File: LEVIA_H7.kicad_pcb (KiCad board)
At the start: 6 copper layers, 36.7 x 36.7 mm, 145 parts, among them J1 TF-028-H265, Q1 AO3400A, SW1 SW_Push, U1 USBLC6-2P6, U10 ZX-SH1.0-4PWT, U11 ZX-SH1.0-3PWT, U12 SIT1051TK/3, U13 ZX-SH1.0-4PWT, U14 ICM-42688-P, U15 ICM-42688-P, U16 DPS368XTSA1, U17 IST8310, U18 ZX-SH1.0-4PWT, U19 ZX-SH1.0-6PWT, U2 STM32H743VIHx, U20 ZX-SH1.0-6PWT, U21 ZX-SH1.0-3PWT, U22 ZX-SH1.0-8PWT, U24 ZX-SH1.0-4PWT, U25 BME680, U3 ZX-SH1.0-4PWT, U4 LMR43620R5RPER, U5 LMR604303SRAKRQ1, U6 AP7361C-33FGE-7, U7 AP7361C-33FGE-7, U8 ZX-SH1.0-4PWT, U9 AT7456ELAH, Y1 8MHz, Y2 XL7EL89COI-111YLC-27M

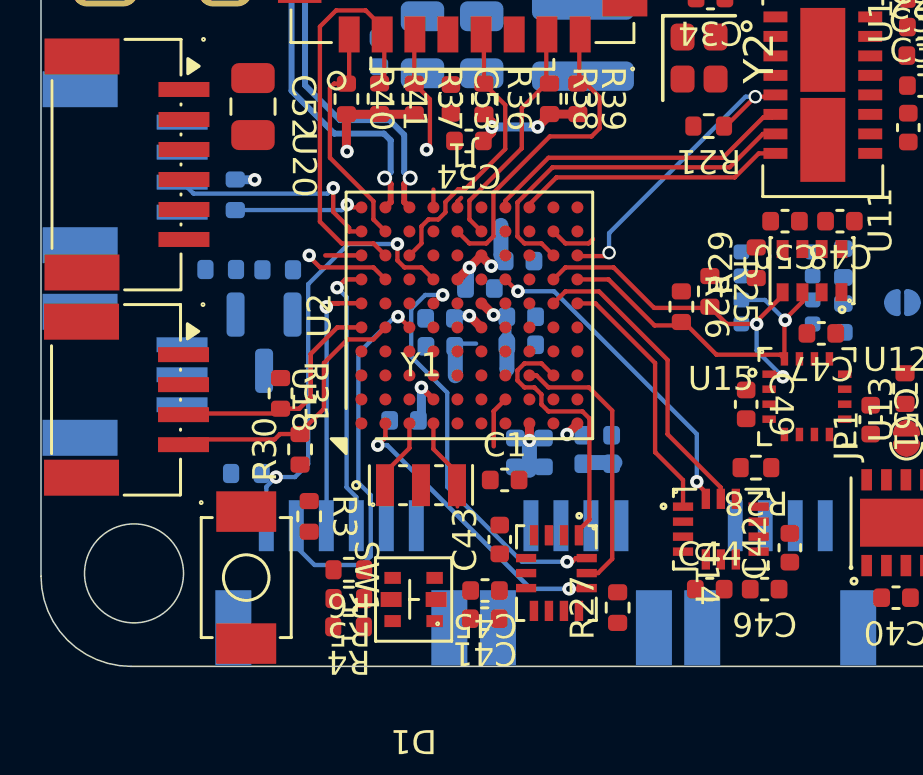
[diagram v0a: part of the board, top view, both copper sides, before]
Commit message: save
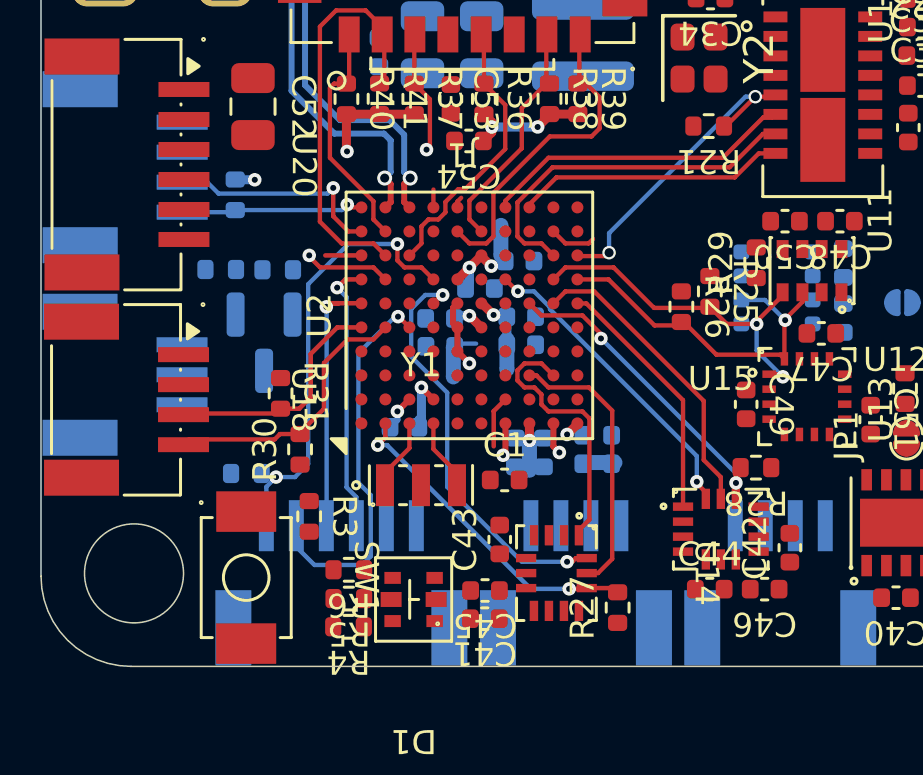
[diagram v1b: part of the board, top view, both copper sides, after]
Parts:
- moved C6 0.23 mm to (132.6, 79.6)
- moved NT4 0.08 mm to (134.2, 77.4)
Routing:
- net /MCU/SPI4.CS: track 0.00 -> 10.7 mm, vias 0 -> 2
- net GND: track 0.00 -> 5.63 mm, vias 0 -> 4
- net /MCU/SWDIO: track 4.32 -> 6.12 mm
- net /MCU/SPI1.CS: track 9.79 -> 10.9 mm
- net /MCU/VDD: track 12.8 -> 13.6 mm
